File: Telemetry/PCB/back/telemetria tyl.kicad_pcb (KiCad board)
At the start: 2 copper layers, 89 parts, among them IC1 LM741CN_NOPB, IC2 LM741CN_NOPB, IC3 LM741CN_NOPB, IC4 NCX2200GW,125, J1 Conn_01x26_Male, J2 Conn_02x05_Odd_Even, Q1 PMF250XNEX, U1 STM32F405RGTx, U2 MCP2561-E-SN, Y1 Crystal_GND24_Small

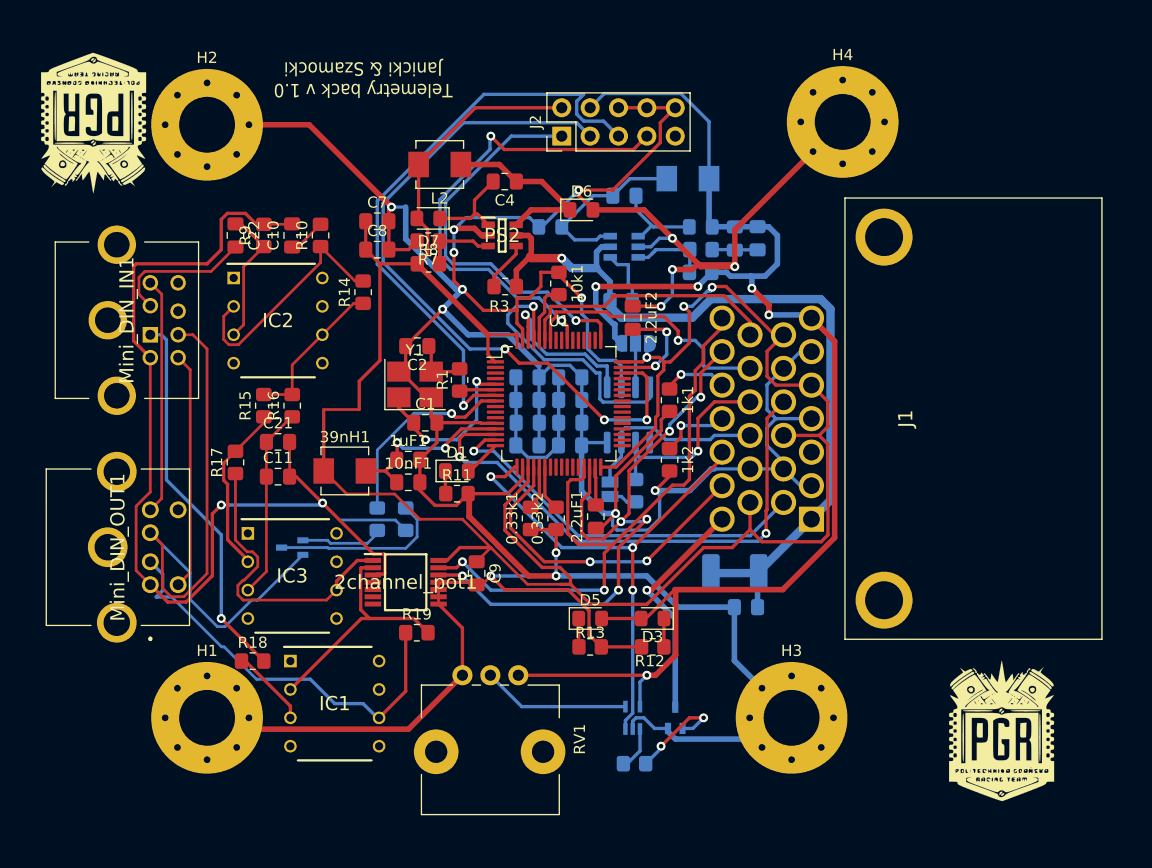
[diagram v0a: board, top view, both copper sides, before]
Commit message: finnal
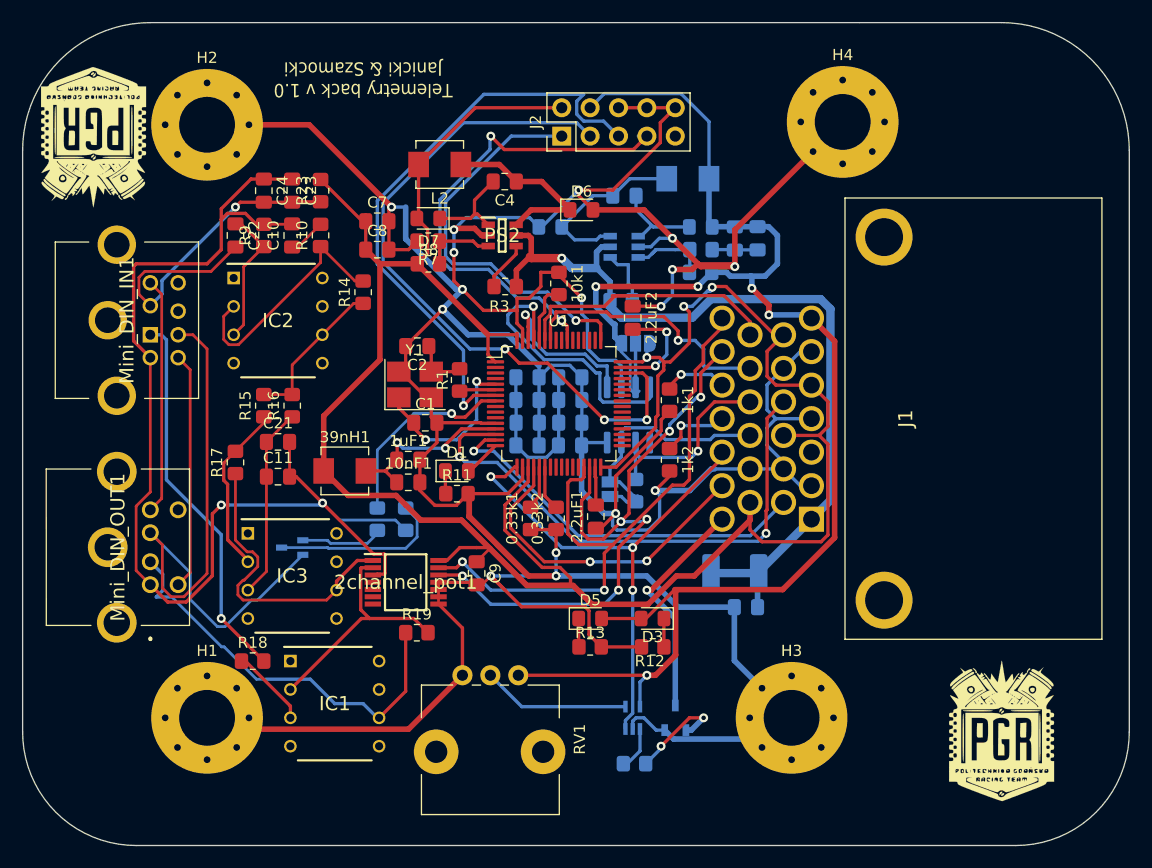
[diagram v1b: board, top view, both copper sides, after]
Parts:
- added C23: ?, Capacitor_SMD:C_0805_2012Metric_Pad1.18x1.45mm_HandSolder, F.Cu at (43.2, 31.6)
- added C24: 10uF, Capacitor_SMD:C_0805_2012Metric_Pad1.18x1.45mm_HandSolder, F.Cu at (40.6, 31.6)
- added R23: R, Resistor_SMD:R_0805_2012Metric_Pad1.20x1.40mm_HandSolder, F.Cu at (45.7, 31.6)
- Q1: value PMF250XNEX -> PMV280ENEAR; footprint SamacSys_Parts:PMF250XNEX -> SamacSys_Parts:PMV280ENEAR
- R4: value R -> 120
- moved G*** 1.27 mm to (25.4, 26.7)
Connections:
- R4 pad 1: Net-(JP2-Pad1) -> CAN_H1
- U2 pad 3: Net-(JP1-Pad2) -> +5V
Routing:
- net +3V3: track 227.3 -> 268.3 mm
- net V_ANC: track 12.7 -> 32.5 mm, vias 0 -> 1
- net GND_MIC&ANC: track 97.3 -> 105.7 mm
- net +5V: track 134.2 -> 139.7 mm
- net CAN_H1: track 17.2 -> 20.4 mm
- net GND: track 444.3 -> 445.9 mm
- net Net-(Q1-Pad1): track 9.28 -> 10.4 mm
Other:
- board outline added: 99.1 x 73.7 mm
